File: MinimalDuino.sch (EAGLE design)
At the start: 16 parts, among them J1 AVR_SPI_PRG_6PTH, U1 ATMEGA328P

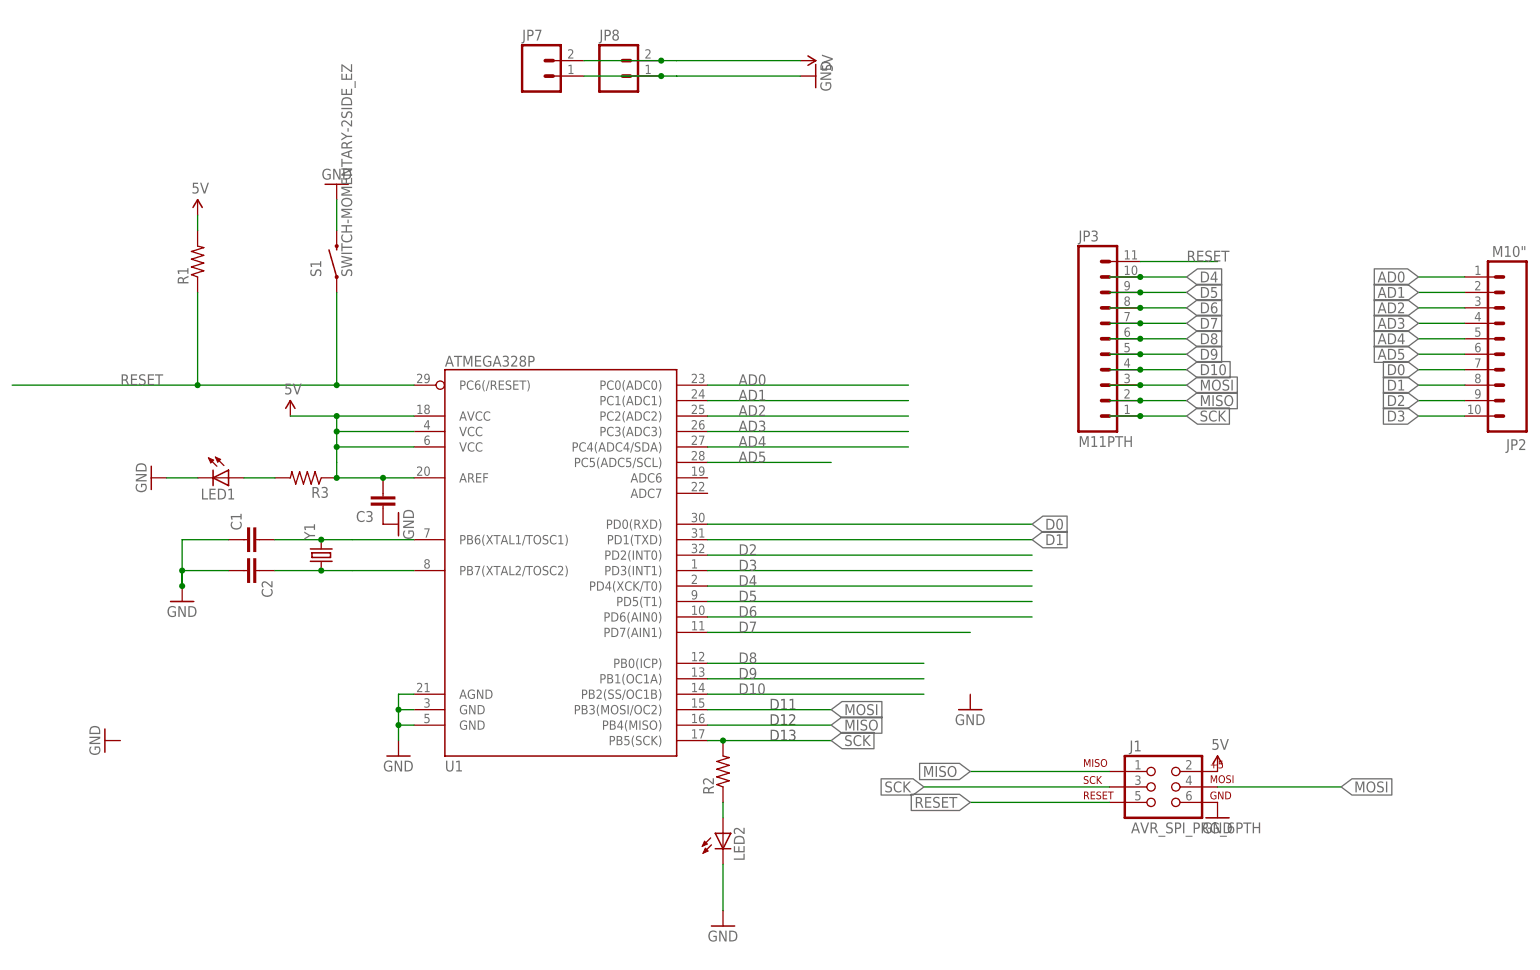
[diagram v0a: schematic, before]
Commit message: Board and schematic updates
Board and schematic updates
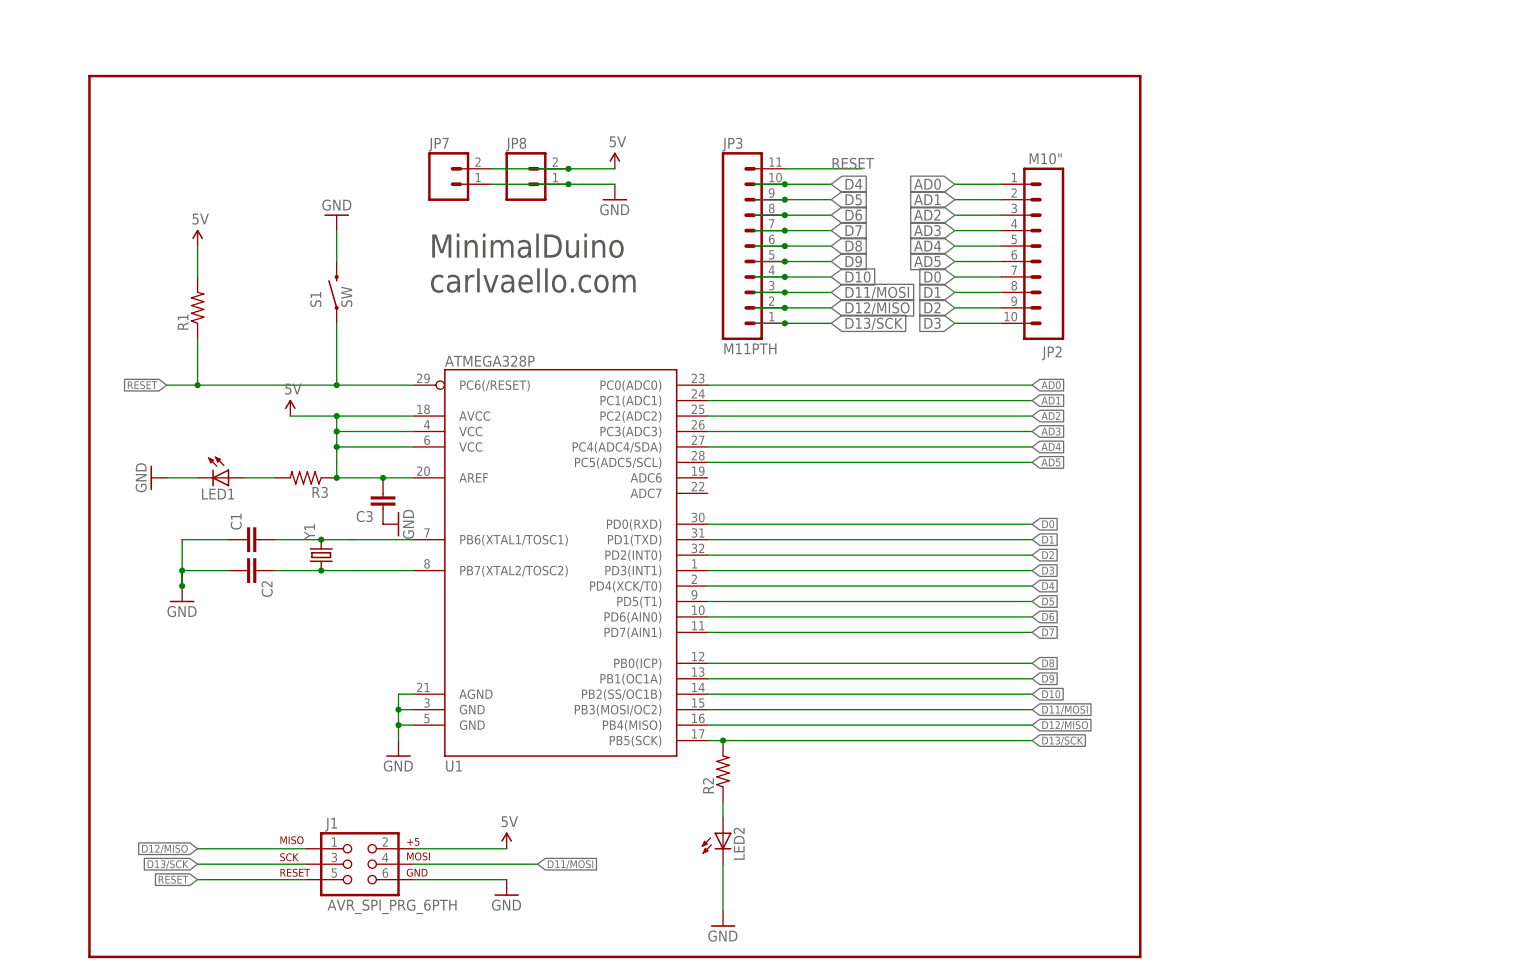
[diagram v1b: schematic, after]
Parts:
- S1: value SWITCH-MOMENTARY-2SIDE_EZ -> SW
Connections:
- net MISO renamed D12/MISO
- net MOSI renamed D11/MOSI
- net SCK renamed D13/SCK
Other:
- note added: "MinimalDuino carlvaello.com"
- note removed: "D11"
- note removed: "D12"
- note removed: "D13"
- moved on the sheet: J1, JP2, JP3, JP7, JP8, R1, S1
